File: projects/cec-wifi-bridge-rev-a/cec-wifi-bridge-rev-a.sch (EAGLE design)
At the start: 54 parts, among them J1 DX4R005H91R1500, J3 DEBUG, J4 10029449-001RLF, J5 PROGRAM, T1 MMBT3904, T2 MMBT3904, U1 MCP73831/2/OT, U2 TPS61200DRC, U3 ESP8266EX, U4 SPI-FLASH-SOIC8, X1 26MHz

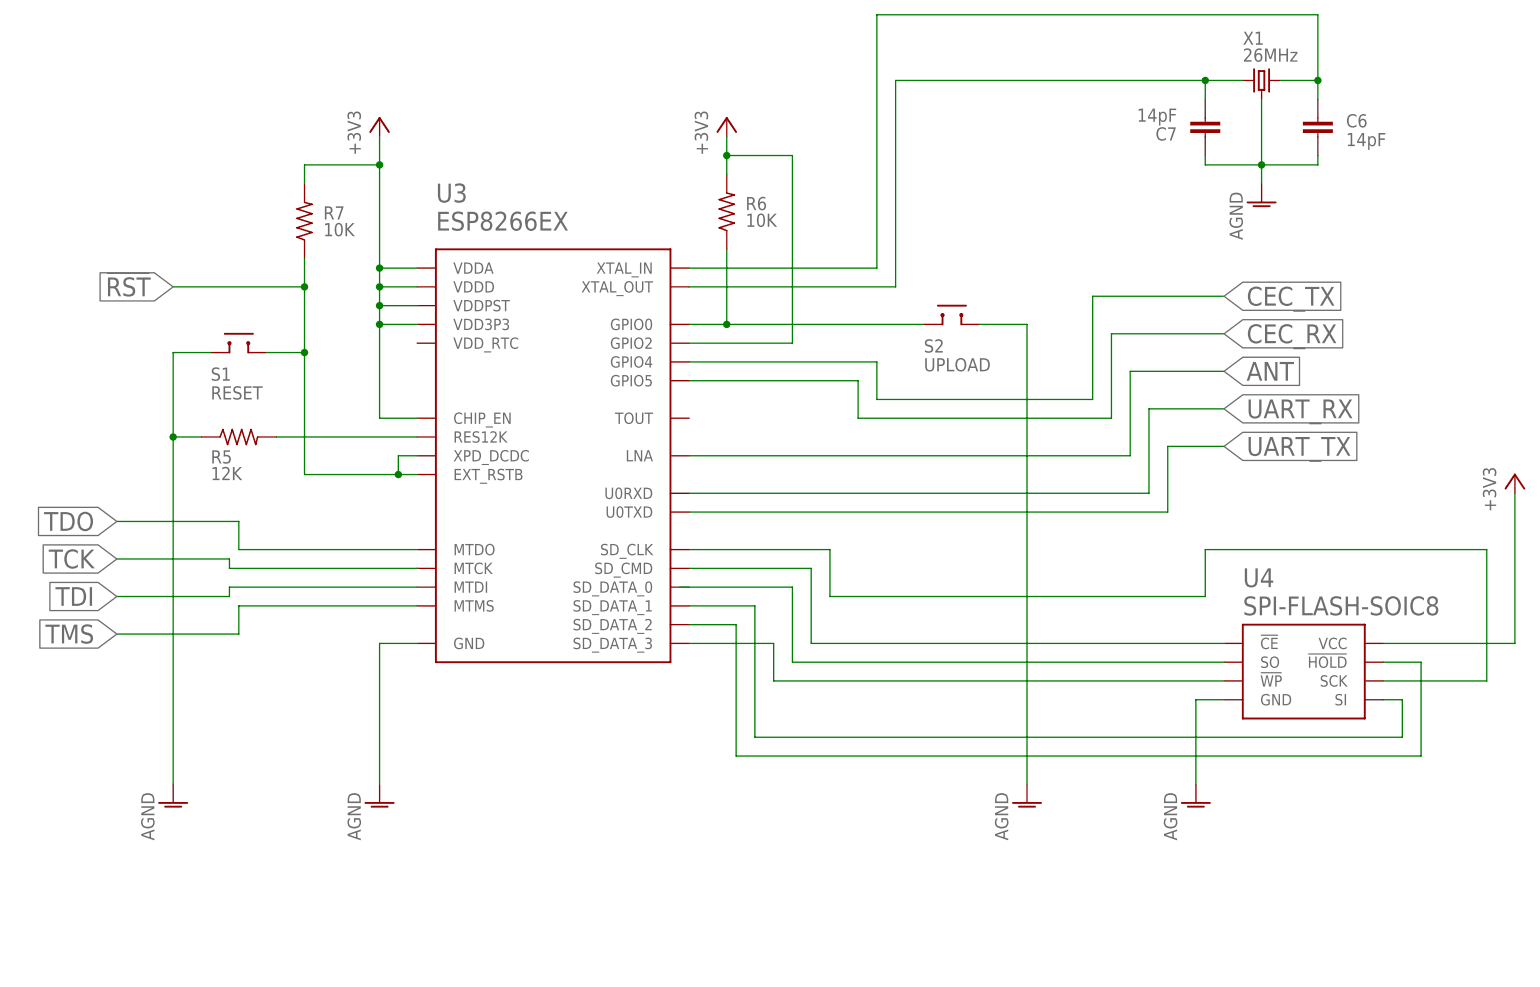
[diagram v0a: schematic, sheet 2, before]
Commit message: cleanup
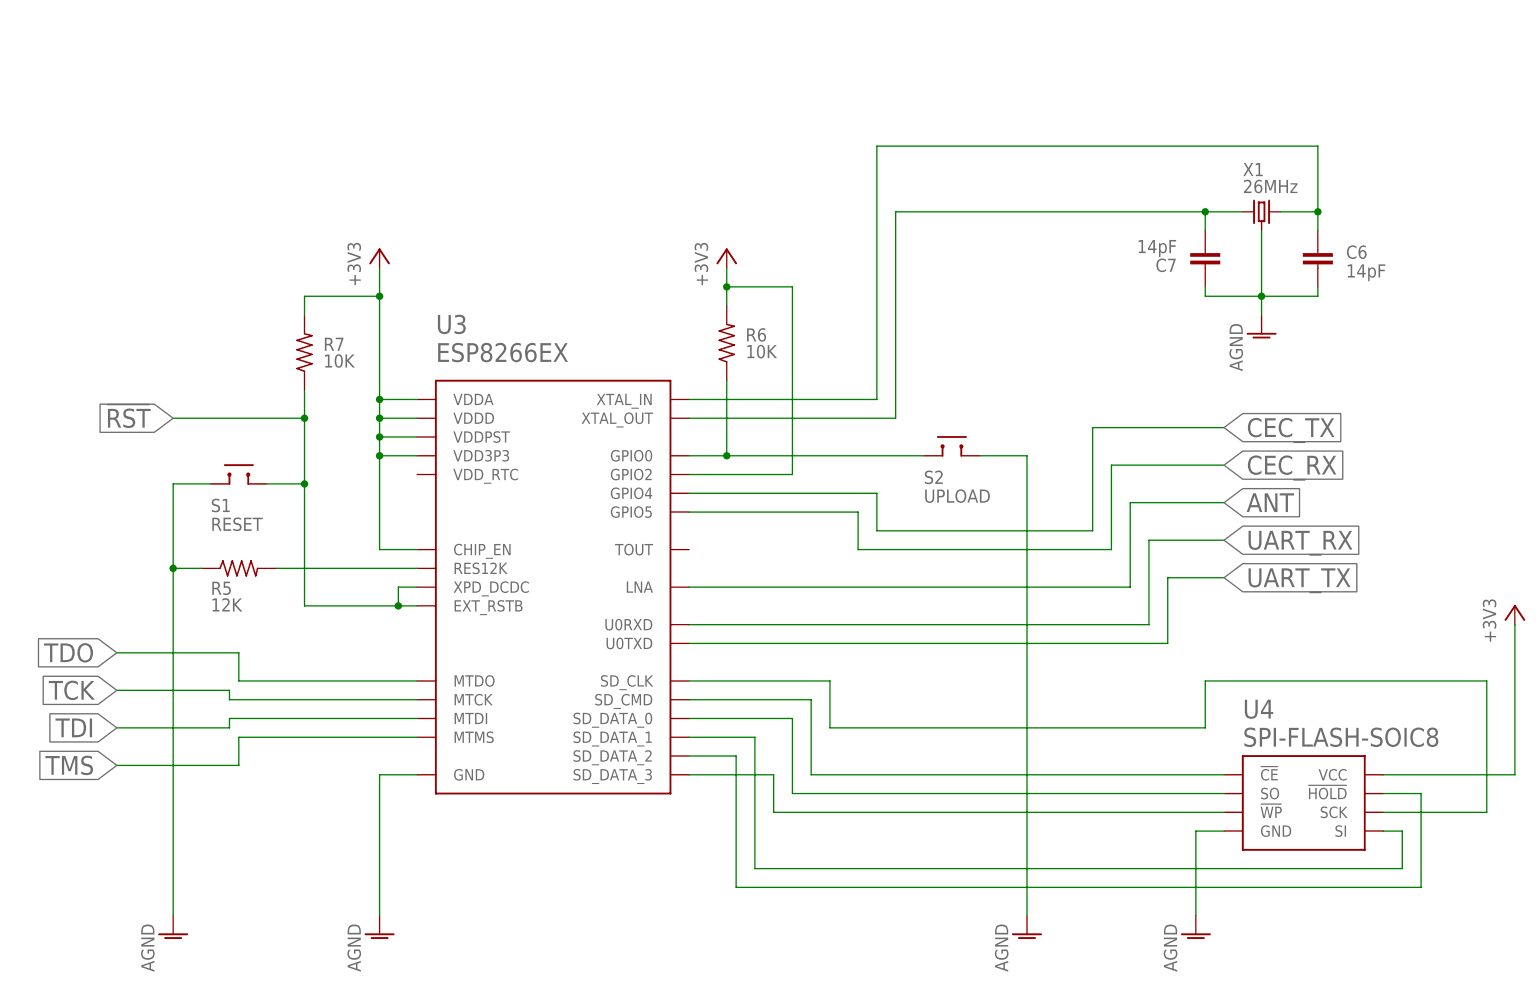
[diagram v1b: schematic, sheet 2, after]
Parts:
- ANT1, J2: BOM (none) -> EXCLUDE
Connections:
- net N$23: now also U3.SD_DATA_0
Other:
- note added: "CEC Interface / Demux"
- note added: "CEC is a one-wire bidirectional protocol, so this circuit allows us to break out the TX and RX into separate lines to allow for an easy software-based implementation."
- note added: "We're using the ESP8266 here to provide simple and effective WiFI control."
- note added: "WiFi / CEC Control"
- moved on the sheet: C17, C6, C7, D2, R10, R11, R12, R13, R14, R15, R5, R6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
